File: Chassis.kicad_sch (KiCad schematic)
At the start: 10 parts, among them J1 Conn_01x02, J10 Conn_01x02, J2 Conn_01x02, J3 Conn_01x02, J4 Conn_01x02, J5 Conn_01x02, J6 Conn_01x02, J7 Conn_01x02, J8 Conn_01x02, J9 Conn_01x02

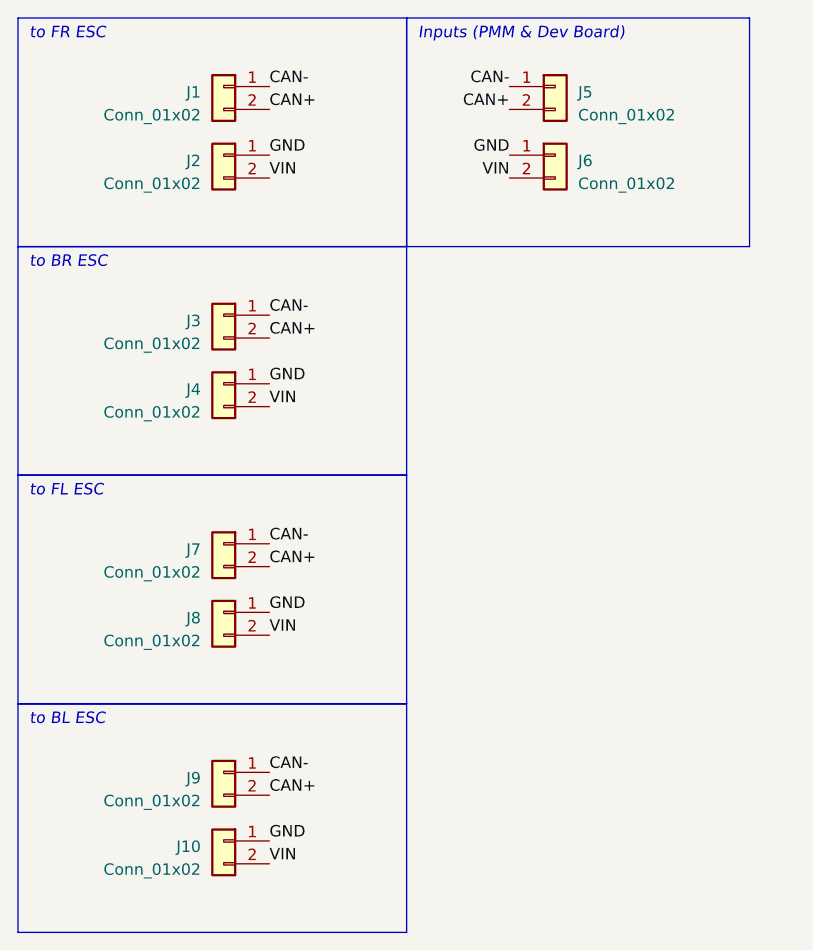
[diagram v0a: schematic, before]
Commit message: Possible indicator method?
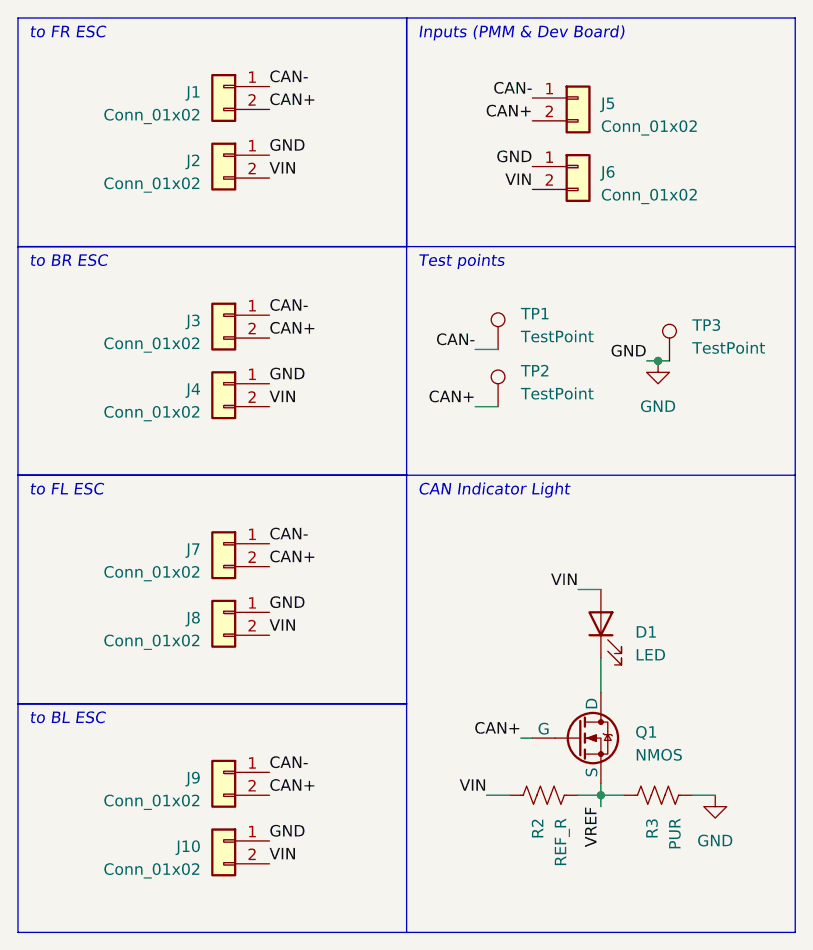
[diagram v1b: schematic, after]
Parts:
- added D1: LED, symbol Device:LED
- added Q1: NMOS, symbol Simulation_SPICE:NMOS
- added R2: REF_R, Resistor_SMD:R_0603_1608Metric_Pad0.98x0.95mm_HandSolder, symbol Device:R_US
- added R3: PUR, Resistor_SMD:R_0603_1608Metric_Pad0.98x0.95mm_HandSolder, symbol Device:R_US
- added TP1, TP2, TP3: TestPoint, TestPoint:TestPoint_Pad_1.0x1.0mm, symbol Connector:TestPoint
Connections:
- net CAN+: now also Q1.2 (G), TP2.1
- net CAN-: now also TP1.1
- net GND: now also R3.2, TP3.1
- net VIN: now also D1.2 (A), R2.1
- new net: D1.1 (K), Q1.1 (D)
- new net VREF: Q1.3 (S), R2.2, R3.1
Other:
- note added: "CAN Indicator Light"
- note added: "Test points"
- moved on the sheet: J5, J6
